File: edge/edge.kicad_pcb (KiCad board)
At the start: 2 copper layers, 50 x 50 mm, 22 parts, among them IC1 ATTINY861A-S, P1 CONN_6, P2 CONN_6, P3 CONN_5, P4 CONN_6, P5 CONN_3X2, Q1 MOSFET_N, Q2 MOSFET_N, Q3 MOSFET_N

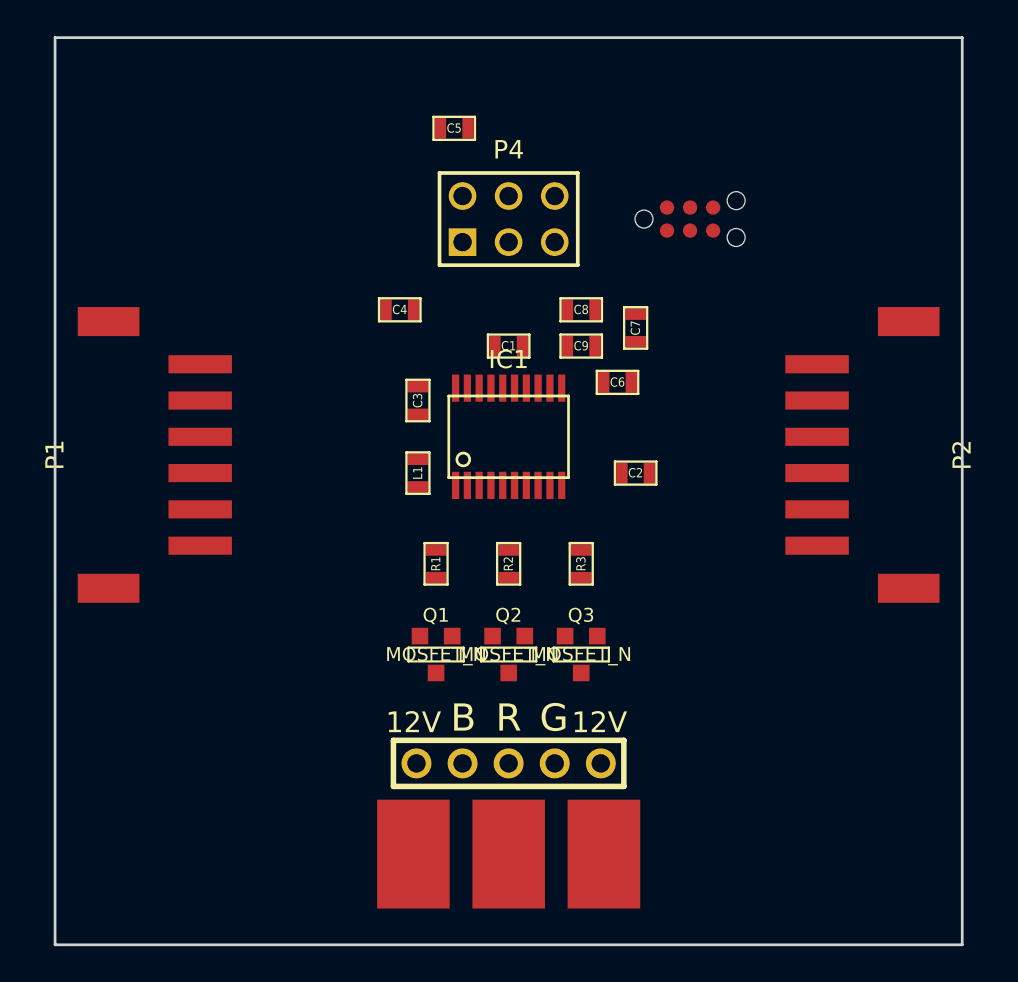
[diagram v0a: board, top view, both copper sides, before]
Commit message: Last version before ATtiny24A
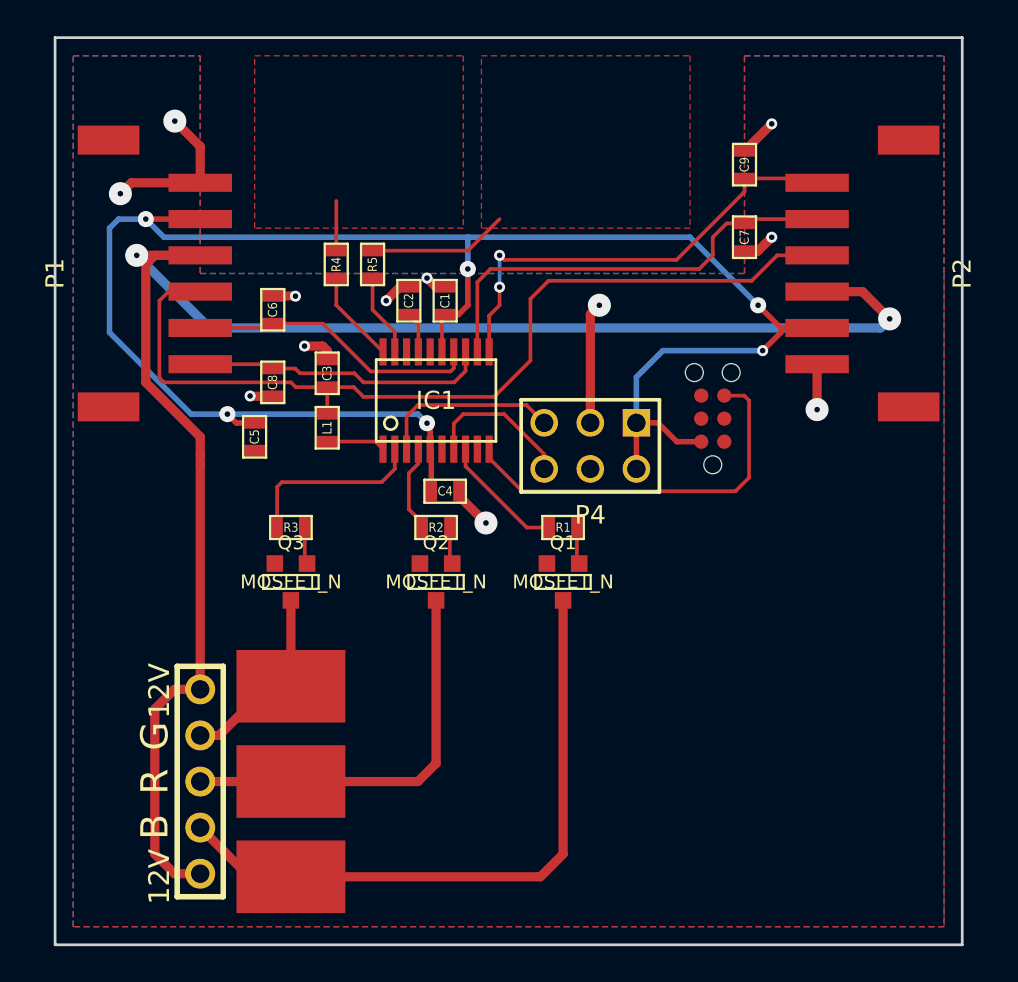
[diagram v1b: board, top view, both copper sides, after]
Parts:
- added R4: 10K, SM0603, F.Cu at (215.5, 112.5)
- added R5: 10K, SM0603, F.Cu at (217.5, 112.5)
- moved C5 20.2 mm to (211.0, 122.0), turned to 270 degrees
- moved C6 19.4 mm to (212.0, 115.0), turned to 90 degrees
- moved C8 17.5 mm to (212.0, 119.0), turned to 270 degrees
- moved P3 17.0 mm to (208.0, 141.0), turned to 90 degrees
- moved Q3 16.5 mm to (213.0, 130.0)
- moved R3 16.1 mm to (213.0, 127.0), turned to 0 degrees
- moved C2 15.7 mm to (219.5, 114.5), turned to 90 degrees
- moved C9 13.5 mm to (238.0, 107.0), turned to 90 degrees
- moved P4 13.3 mm to (229.5, 122.5), turned to 180 degrees
- moved P5 11.1 mm to (236.2, 121.0), turned to 90 degrees
- moved C4 10.3 mm to (221.5, 125.0)
- moved P1 10.0 mm to (208.0, 113.0)
- moved P2 10.0 mm to (242.0, 113.0)
- moved Q1 8.06 mm to (228.0, 130.0)
- moved C7 7.81 mm to (238.0, 111.0), turned to 270 degrees
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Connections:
- C3 pad 2: N-000007 (its old number) -> /OUT
- IC1 pad 1: /OUT -> /MOSI
- IC1 pad 19: N-0000019 (its old number) -> /BTN2
- IC1 pad 2: /RED -> /BLUE
- IC1 pad 20: /PA0 -> /BTN1
- IC1 pad 3: N-000004 -> /PB2
- IC1 pad 7: N-000005 -> /PB4
- IC1 pad 8: /BLUE -> /RED
- L1 pad 1: /OUT -> /MOSI
- L1 pad 2: N-000007 (its old number) -> /OUT
- P4 pad 5: /PA0 -> /PB2
- P4 pad 6: /PA2 -> /PB4
- P5 pad 1: /MISO -> /BLUE
- P5 pad 3: /SCK -> /PB2
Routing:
- net +3.3V: track 0.00 -> 101.2 mm, vias 0 -> 6
- net +12V: track 0.00 -> 93.2 mm, vias 0 -> 2
- net /OUT: track 0.00 -> 50.1 mm
- net N-000001: track 0.00 -> 35.6 mm
- net GND: track 0.00 -> 31.6 mm, vias 0 -> 12
- net /INCCW2: track 0.00 -> 25.6 mm, vias 0 -> 2
- net /INCW2: track 0.00 -> 24.6 mm
- net N-0000018: track 0.00 -> 22.4 mm
- net /\RESET: track 0.00 -> 21.6 mm
- net /INCCW1: track 0.00 -> 16.4 mm
- net /INCW1: track 0.00 -> 16.1 mm
- net N-0000019: track 0.00 -> 10.9 mm
- net /BLUE: track 0.00 -> 10.2 mm
- net /PB2: track 0.00 -> 10.1 mm
- net /PB4: track 0.00 -> 8.33 mm
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- added copper zone on F.Cu, net /BTN1C
- added copper zone on F.Cu, net /BTN2C
- added copper zone on B.Cu, net GND
- added copper zone on F.Cu, net GND
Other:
- net class Default: clearance 0.254 -> 0.2032; trace_width 0.254 -> 0.2032; via_dia 0.889 -> 0.6096; via_drill 0.635 -> 0.3048
- net class hipower added: clearance 0.3048, trace_width 0.508, via_dia 1.27, via_drill 0.762
- net class power added: clearance 0.2032, trace_width 0.3048, via_dia 0.889, via_drill 0.508
- rule trace_clearance: 0.254 -> 0.2032
- rule trace_min: 0.254 -> 0.1524
- rule via_min_drill: 0.508 -> 0.3048
- rule via_min_size: 0.889 -> 0.6096
